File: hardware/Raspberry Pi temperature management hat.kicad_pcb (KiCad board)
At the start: 2 copper layers, 65 x 56 mm, 28 parts, among them J1 Screw Terminal x3, J2 Screw Terminal x2, J3 OX40HAT, Q1 S8050, U1 MIC5225-3.3, U2 MAX31865, U3 LTV-817S

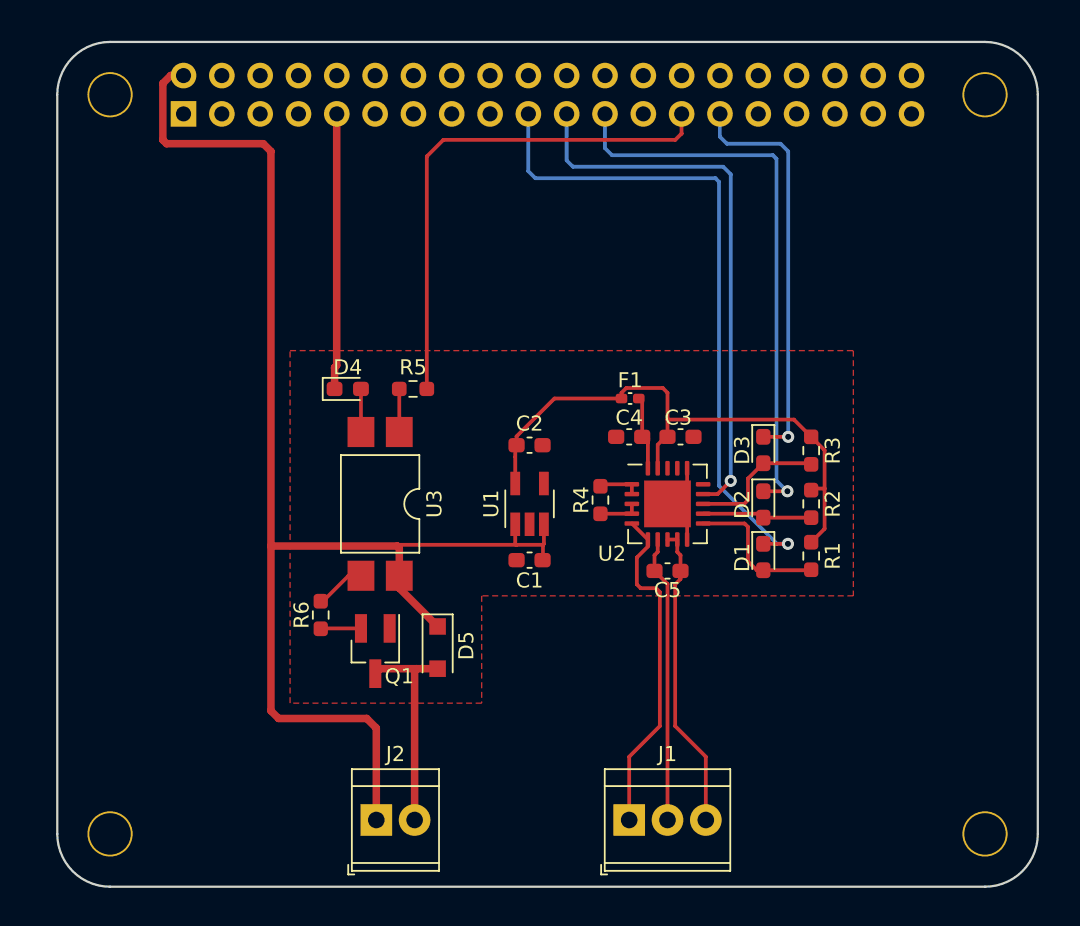
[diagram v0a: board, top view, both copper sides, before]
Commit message: PCB board V2
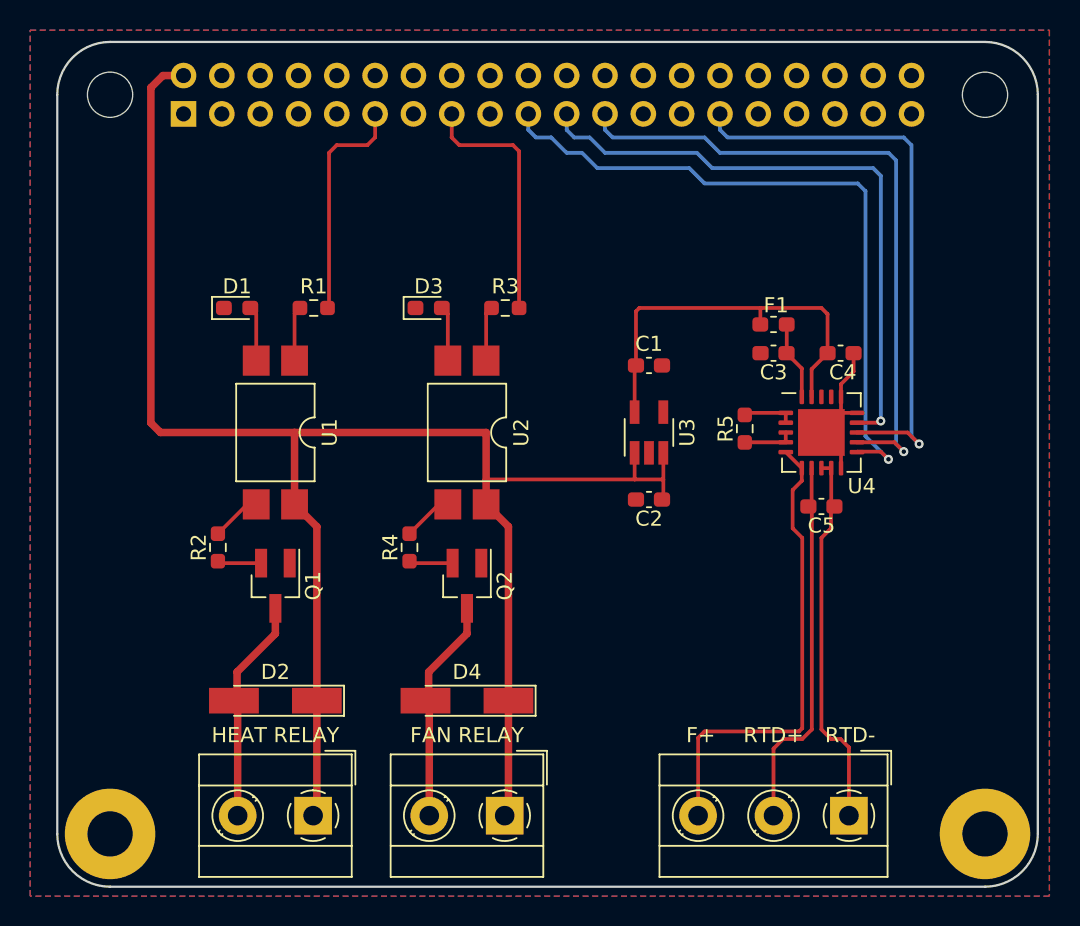
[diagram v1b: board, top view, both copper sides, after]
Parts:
- removed D5: S1MFL, Diode_SMD:D_SOD-123F
- removed R6: 510, Resistor_SMD:R_0603_1608Metric_Pad0.98x0.95mm_HandSolder
- added J3: Screw Terminal x3, TerminalBlock_MetzConnect:TerminalBlock_MetzConnect_Type055_RT01503HDWU_1x03_P5.00mm_Horizontal, F.Cu at (99.0, 97.8)
- added Q2: S8050, Package_TO_SOT_SMD:SOT-23_Handsoldering, F.Cu at (73.7, 82.5)
- added U4: MAX31865, Package_DFN_QFN:TQFN-20-1EP_5x5mm_P0.65mm_EP3.1x3.1mm, F.Cu at (97.2, 72.4)
- C1: value 10uF -> 0.1uF
- C4: value 0.1uF -> 10uF
- D1, D3: value 1N4148W -> LED; footprint Diode_SMD:D_0603_1608Metric_Pad1.05x0.95mm_HandSolder -> LED_SMD:LED_0603_1608Metric_Pad1.05x0.95mm_HandSolder
- D2: value 1N4148W -> LL4148; footprint Diode_SMD:D_0603_1608Metric_Pad1.05x0.95mm_HandSolder -> Diode_SMD:D_MiniMELF_Handsoldering
- D4: value LED -> LL4148; footprint LED_SMD:LED_0603_1608Metric_Pad1.05x0.95mm_HandSolder -> Diode_SMD:D_MiniMELF_Handsoldering
- F1: footprint Fuse:Fuse_0402_1005Metric_Pad0.77x0.64mm_HandSolder -> Fuse:Fuse_0603_1608Metric_Pad1.05x0.95mm_HandSolder
- H1, H2: value 3mm_Mounting_Hole -> MountingHole; footprint project_footprints:NPTH_3mm_ID -> MountingHole:MountingHole_3mm
- H3, H4: value 3mm_Mounting_Hole -> MountingHole_Pad; footprint project_footprints:NPTH_3mm_ID -> MountingHole:MountingHole_3mm_Pad
- J1: value Screw Terminal x3 -> Screw Terminal x2; footprint TerminalBlock_TE-Connectivity:TerminalBlock_TE_282834-3_1x03_P2.54mm_Horizontal -> TerminalBlock_MetzConnect:TerminalBlock_MetzConnect_Type055_RT01502HDWU_1x02_P5.00mm_Horizontal
- J2: footprint TerminalBlock_TE-Connectivity:TerminalBlock_TE_282834-2_1x02_P2.54mm_Horizontal -> TerminalBlock_MetzConnect:TerminalBlock_MetzConnect_Type055_RT01502HDWU_1x02_P5.00mm_Horizontal
- R1, R3: value 10k -> 180
- R2: value 10k -> 510
- R4: value 430, 0.1% -> 510
- R5: value 180 -> 430, 0.1%
- U1: value MIC5225-3.3 -> LTV-817S; footprint Package_TO_SOT_SMD:SOT-23-5_HandSoldering -> Package_DIP:SMDIP-4_W9.53mm
- U2: value MAX31865 -> LTV-817S; footprint Package_DFN_QFN:TQFN-20-1EP_5x5mm_P0.65mm_EP3.1x3.1mm -> Package_DIP:SMDIP-4_W9.53mm
- U3: value LTV-817S -> MIC5225-3.3; footprint Package_DIP:SMDIP-4_W9.53mm -> Package_TO_SOT_SMD:SOT-23-5_HandSoldering
- moved R2 39.4 mm to (57.1, 80.0)
- moved D1 38.6 mm to (58.4, 64.1), turned to 0 degrees
- moved R1 36.8 mm to (63.5, 64.1), turned to 0 degrees
- moved D2 34.9 mm to (61.0, 90.2), turned to 180 degrees
- moved D3 24.1 mm to (71.1, 64.1), turned to 0 degrees
- moved R3 22.4 mm to (76.2, 64.1), turned to 0 degrees
- moved R5 22.1 mm to (92.1, 72.1), turned to -90 degrees
- moved D4 22.1 mm to (73.7, 90.2), turned to 180 degrees
- moved J1 21.0 mm to (63.5, 97.8), turned to 180 degrees
- moved U3 18.4 mm to (85.7, 72.4), turned to 90 degrees
- moved U1 17.5 mm to (61.0, 72.4), turned to -90 degrees
- moved C1 15.1 mm to (85.7, 67.9)
- moved C4 15.1 mm to (98.4, 67.1)
- moved U2 14.1 mm to (73.7, 72.4), turned to -90 degrees
- moved R4 13.0 mm to (69.8, 80.0)
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- renumbered J3 to J4
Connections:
- C1 pad 1: GND -> VDD
- C1 pad 2: +5V -> GND
- C2 pad 1: VDD -> GND
- C2 pad 2: GND -> +5V
- C3 pad 1: VDD -> GND
- C3 pad 2: GND -> Net-(C3-Pad2)
- C4 pad 1: GND -> VDD
- C4 pad 2: Net-(C4-Pad2) -> GND
- D1 pad 1: /SDI -> GND
- D2 pad 1: /SCLK -> +5V
- D3 pad 1: /CS -> GND
- D4 pad 1: GND -> +5V
- F1 pad 1: Net-(C4-Pad2) -> Net-(C3-Pad2)
- J1 pad 1: Net-(J1-Pad1) -> +5V
- J1 pad 2: Net-(C5-Pad1) -> Net-(D2-Pad2)
- J2 pad 2: Net-(D5-Pad2) -> Net-(D4-Pad2)
- J4 pad 11: unconnected-(J3-Pad11) -> /HET
- J4 pad 15: unconnected-(J3-Pad15) -> /FAN
- J4 pad 27: /REL -> unconnected-(J4-Pad27)
- J4 pad 39: unconnected-(J3-Pad39) -> GND
- J4 pad 9: GND -> unconnected-(J4-Pad9)
- Q1 pad 3: Net-(D5-Pad2) -> Net-(D2-Pad2)
- R1 pad 1: VDD -> Net-(R1-Pad1)
- R1 pad 2: Net-(D1-Pad2) -> /HET
- R2 pad 1: VDD -> Net-(R2-Pad1)
- R2 pad 2: Net-(D2-Pad2) -> Net-(Q1-Pad2)
- R3 pad 1: VDD -> Net-(R3-Pad1)
- R3 pad 2: Net-(D3-Pad2) -> /FAN
- R4 pad 2: Net-(R4-Pad2) -> Net-(Q2-Pad2)
- R5 pad 2: /REL -> Net-(R5-Pad2)
- U1 pad 1: +5V -> Net-(R1-Pad1)
- U1 pad 2: GND -> Net-(D1-Pad2)
- U1 pad 3: +5V -> Net-(R2-Pad1)
- U1 pad 4: unconnected-(U1-Pad4) -> +5V
- U2 pad 1: Net-(R4-Pad1) -> Net-(R3-Pad1)
- U2 pad 2: Net-(R4-Pad1) -> Net-(D3-Pad2)
- U2 pad 3: Net-(R4-Pad2) -> Net-(R4-Pad1)
- U2 pad 4: Net-(R4-Pad2) -> +5V
- U3 pad 1: Net-(R5-Pad1) -> +5V
- U3 pad 2: Net-(D4-Pad2) -> GND
- U3 pad 3: Net-(R6-Pad1) -> +5V
- U3 pad 4: +5V -> unconnected-(U3-Pad4)
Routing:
- net /REL: track 34.2 -> 0.00 mm
- net Net-(J3-Pad3): track 0.00 -> 31.6 mm
- net +5V: track 91.8 -> 116.1 mm
- net Net-(J1-Pad1): track 22.5 -> 0.00 mm
- net /FAN: track 0.00 -> 16.8 mm
- net /HET: track 0.00 -> 15.4 mm
- net Net-(D5-Pad2): track 14.3 -> 0.00 mm
- net GND: track 24.4 -> 10.4 mm
- net VDD: track 38.8 -> 26.7 mm
- net Net-(D4-Pad2): track 2.86 -> 15.0 mm
- net /CS: track 27.0 -> 38.6 mm
- net Net-(D2-Pad2): track 7.27 -> 15.0 mm
- net Net-(C5-Pad1): track 19.0 -> 25.3 mm
- net /SCLK: track 37.9 -> 44.1 mm
- net Net-(D1-Pad2): track 9.80 -> 3.65 mm
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- added copper zone on B.Cu, net GND
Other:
- board text added: "F+"
- board text added: "FAN RELAY"
- board text added: "HEAT RELAY"
- board text added: "RTD+"
- board text added: "RTD-"
